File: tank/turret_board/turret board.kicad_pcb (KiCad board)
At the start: 2 copper layers, 69 x 39 mm, 22 parts, among them P1 Power, P2 IR Beacon, P3 SigIn, P4 IR Tx, P5 IR Rx, U1 LM317T, U2 pixart_ir, Y1 Crystal_4pin

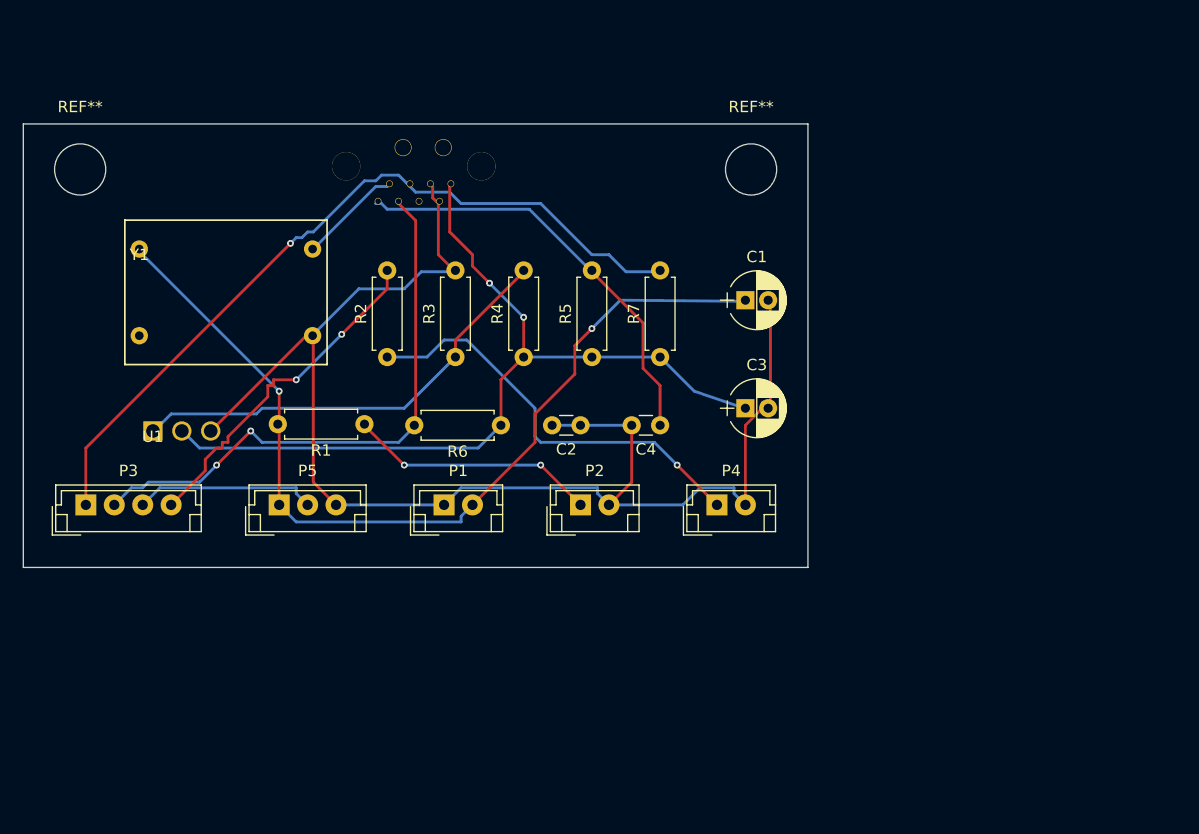
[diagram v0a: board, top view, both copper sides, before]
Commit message: main board v0.1
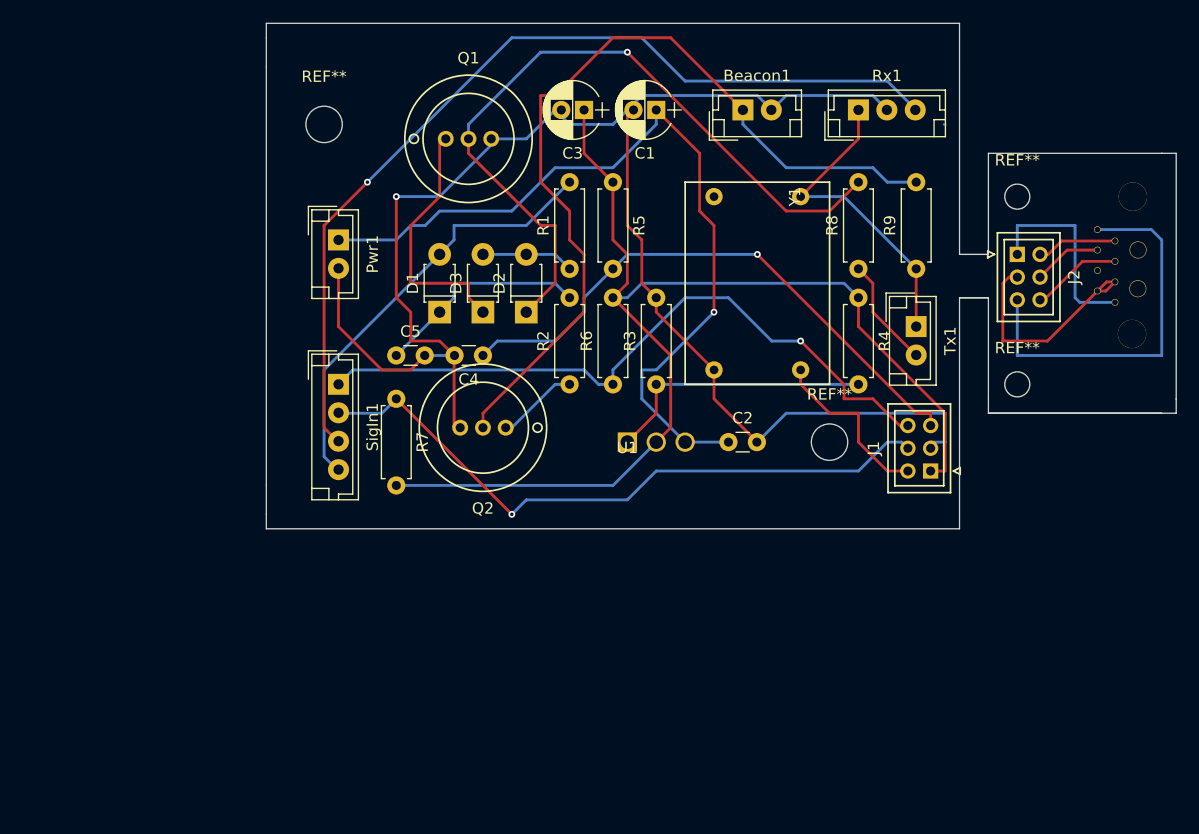
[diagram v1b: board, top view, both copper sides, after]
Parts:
- removed ?: , Tank:MIAR
- removed P1: Power, JST:JST_EH_B02B-EH-A_02x2.50mm_Straight
- removed P2: IR Beacon, JST:JST_EH_B02B-EH-A_02x2.50mm_Straight
- removed P3: SigIn, JST:JST_EH_B04B-EH-A_04x2.50mm_Straight
- removed P4: IR Tx, JST:JST_EH_B02B-EH-A_02x2.50mm_Straight
- removed P5: IR Rx, JST:JST_EH_B03B-EH-A_03x2.50mm_Straight
- removed the REF** at (150.0, 70.0)
- removed the REF** at (209.0, 70.0)
- added Beacon1: CONN_01X02, JST:JST_EH_B02B-EH-A_02x2.50mm_Straight, F.Cu at (208.3, 64.8)
- added C5: C, Capacitors_THT:C_Disc_D3.0mm_W1.6mm_P2.50mm, F.Cu at (177.8, 86.4)
- added D1: D, Diodes_THT:D_T-1_P5.08mm_Horizontal, F.Cu at (181.6, 82.5)
- added D2: D, Diodes_THT:D_T-1_P5.08mm_Horizontal, F.Cu at (189.2, 82.5)
- added D3: D, Diodes_THT:D_T-1_P5.08mm_Horizontal, F.Cu at (185.4, 82.5)
- added G***: LOGO, modules:miar_logo, B.Cu at (182.9, 71.1)
- added J1: Conn_01x06, Connectors_JAE:JAE_LY20-06P-2T_2x03x2.00mm_Straight, F.Cu at (224.8, 96.5)
- added J2: Conn_01x06, Connectors_JAE:JAE_LY20-06P-2T_2x03x2.00mm_Straight, F.Cu at (232.4, 77.5)
- added Pwr1: CONN_01X02, JST:JST_EH_B02B-EH-A_02x2.50mm_Straight, F.Cu at (172.7, 76.2)
- added Q1: Q_NPN_BCE, Transistors_OldSowjetAera:OldSowjetaera_Transistor_Type-I_SmallPads, F.Cu at (184.2, 67.3)
- added Q2: Q_NPN_BCE, Transistors_OldSowjetAera:OldSowjetaera_Transistor_Type-I_SmallPads, F.Cu at (185.4, 92.7)
- added R8: R, Resistors_THT:R_Axial_DIN0207_L6.3mm_D2.5mm_P7.62mm_Horizontal, F.Cu at (218.4, 78.7)
- added R9: R, Resistors_THT:R_Axial_DIN0207_L6.3mm_D2.5mm_P7.62mm_Horizontal, F.Cu at (223.5, 78.7)
- added REF**: MountingHole_2.2mm_M2, Mounting_Holes:MountingHole_2.2mm_M2, F.Cu at (232.4, 72.4)
- added REF**: MountingHole_3.2mm_M3, Mounting_Holes:MountingHole_3.2mm_M3, F.Cu at (171.4, 66.0)
- added REF**: MountingHole_3.2mm_M3, Mounting_Holes:MountingHole_3.2mm_M3, F.Cu at (215.9, 94.0)
- added REF**: MountingHole_2.2mm_M2, Mounting_Holes:MountingHole_2.2mm_M2, F.Cu at (232.4, 88.9)
- added Rx1: CONN_01X03, JST:JST_EH_B03B-EH-A_03x2.50mm_Straight, F.Cu at (218.4, 64.8)
- added SigIn1: CONN_01X04, JST:JST_EH_B04B-EH-A_04x2.50mm_Straight, F.Cu at (172.7, 88.9)
- added Tx1: TX, JST:JST_EH_B02B-EH-A_02x2.50mm_Straight, F.Cu at (223.5, 83.8)
- U2: footprint pixart_ir -> modules:pixart_ir
- moved Y1 58.3 mm to (213.4, 72.4), turned to 270 degrees
- moved U2 54.0 mm to (238.8, 85.1), turned to 0 degrees
- moved U1 41.7 mm to (198.1, 94.0)
- moved R4 29.9 mm to (218.4, 81.3), turned to 270 degrees
- moved C3 29.8 mm to (194.3, 64.8), turned to 180 degrees
- moved R7 23.5 mm to (177.8, 90.2), turned to 270 degrees
- moved R1 22.6 mm to (193.0, 78.7), turned to 90 degrees
- moved C1 18.5 mm to (200.7, 64.8), turned to 180 degrees
- moved R3 17.8 mm to (200.7, 88.9)
- moved C4 16.7 mm to (185.4, 86.4)
- moved R2 16.2 mm to (193.0, 88.9)
- moved R5 15.5 mm to (196.8, 71.1), turned to 270 degrees
- moved C2 13.1 mm to (207.0, 94.0), turned to 0 degrees
- moved R6 10.5 mm to (196.8, 88.9), turned to 90 degrees
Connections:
- C1 pad 2: Net-(C1-Pad2) -> GND
- C2 pad 1: Net-(C1-Pad2) -> Net-(C1-Pad1)
- C2 pad 2: Net-(C1-Pad2) -> GND
- C3 pad 1: +3V3 -> 3.3V
- C3 pad 2: Net-(C1-Pad2) -> GND
- C4 pad 1: Net-(C4-Pad1) -> RESET
- C4 pad 2: Net-(C1-Pad2) -> GND
- R1 pad 2: Net-(C1-Pad1) -> IRSig
- R3 pad 2: Net-(C1-Pad2) -> GND
- R4 pad 1: +3V3 -> 3.3V
- R5 pad 1: +3V3 -> 3.3V
- R5 pad 2: Net-(C4-Pad1) -> RESET
- R6 pad 1: +3V3 -> SLC
- R6 pad 2: Net-(P3-Pad2) -> 3.3V
- R7 pad 1: +3V3 -> SDA
- R7 pad 2: Net-(P3-Pad1) -> 3.3V
- U1 pad 2: +3V3 -> 3.3V
- U1 pad 3: Net-(C1-Pad2) -> Net-(C1-Pad1)
- U2 pad 1: +3V3 -> Net-(J2-Pad1)
- U2 pad 2: Net-(C1-Pad2) -> Net-(J2-Pad2)
- U2 pad 3: Net-(C1-Pad2) -> Net-(J2-Pad2)
- U2 pad 5: Net-(P3-Pad1) -> Net-(J2-Pad6)
- U2 pad 6: Net-(P3-Pad2) -> Net-(J2-Pad5)
- U2 pad 7: Net-(U2-Pad7) -> Net-(J2-Pad4)
- U2 pad 8: Net-(C4-Pad1) -> Net-(J2-Pad3)
- Y1 pad 14: Net-(C1-Pad1) -> 5V
- Y1 pad 7: Net-(C1-Pad2) -> GND
- Y1 pad 8: Net-(U2-Pad7) -> Net-(J1-Pad4)
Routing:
- net GND: track 0.00 -> 151.4 mm, vias 0 -> 1
- net Net-(C1-Pad2): track 127.5 -> 0.00 mm
- net 3.3V: track 0.00 -> 100.7 mm
- net Net-(Rx1-Pad3): track 0.00 -> 81.3 mm, vias 0 -> 1
- net +3V3: track 75.7 -> 0.00 mm, vias 2 -> 0
- net Beacon: track 0.00 -> 75.6 mm
- net Net-(P3-Pad1): track 69.6 -> 0.00 mm, vias 1 -> 0
- net Net-(D2-Pad1): track 0.00 -> 65.2 mm, vias 0 -> 1
- net SLC: track 0.00 -> 60.5 mm, vias 0 -> 1
- net SDA: track 0.00 -> 57.7 mm, vias 0 -> 1
- net Net-(P3-Pad2): track 50.8 -> 0.00 mm, vias 2 -> 0
- net RESET: track 0.00 -> 50.7 mm, vias 0 -> 1
- net IRSig: track 0.00 -> 38.7 mm
- net Net-(C4-Pad1): track 38.0 -> 0.00 mm
- net Net-(J2-Pad3): track 0.00 -> 33.8 mm
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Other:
- board size 69 x 39 mm -> 80 x 44.4 mm
- board text added: "Turret Board v0.3 Laser Tag Robot Tank M.I.A.R. Labs nick.groesz@gmail.com"
- board text removed: "Turret Board v0.2 Laser Bot M.I.A.R. Labs"

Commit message: interim
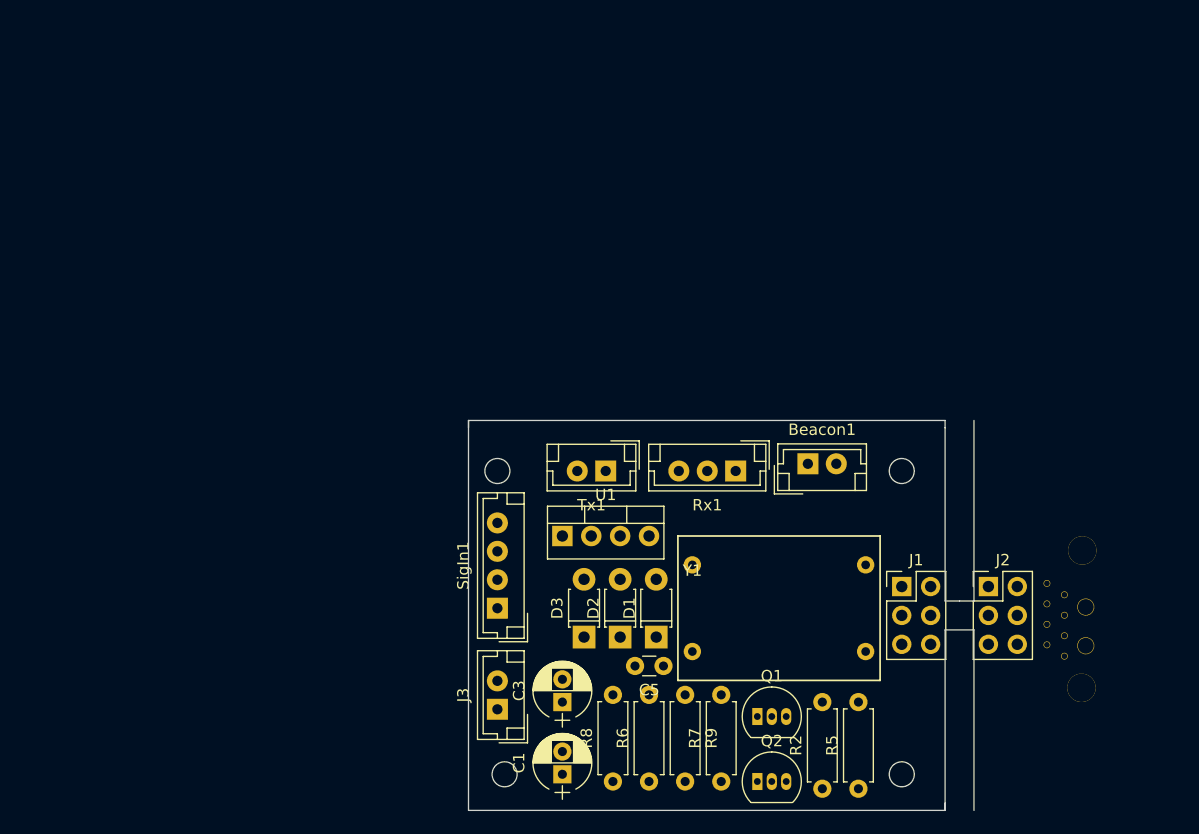
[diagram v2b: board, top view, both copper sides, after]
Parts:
- removed C2, C4: C, Capacitors_THT:C_Disc_D3.0mm_W1.6mm_P2.50mm
- removed G***: LOGO, modules:miar_logo
- removed Pwr1: CONN_01X02, JST:JST_EH_B02B-EH-A_02x2.50mm_Straight
- removed R1, R3, R4: R, Resistors_THT:R_Axial_DIN0207_L6.3mm_D2.5mm_P7.62mm_Horizontal
- removed the REF** at (232.4, 72.4)
- removed the REF** at (171.4, 66.0)
- removed the REF** at (215.9, 94.0)
- removed the REF** at (232.4, 88.9)
- added J3: Conn_01x02_Male, JST:JST_EH_B02B-EH-A_02x2.50mm_Straight, F.Cu at (186.7, 117.5)
- added REF**: MountingHole_2.2mm_M2, Mounting_Holes:MountingHole_2.2mm_M2, F.Cu at (186.7, 96.5)
- added REF**: MountingHole_2.2mm_M2, Mounting_Holes:MountingHole_2.2mm_M2, F.Cu at (187.3, 123.2)
- added REF**: MountingHole_2.2mm_M2, Mounting_Holes:MountingHole_2.2mm_M2, F.Cu at (222.2, 96.5)
- added REF**: MountingHole_2.2mm_M2, Mounting_Holes:MountingHole_2.2mm_M2, F.Cu at (222.2, 123.2)
- J1, J2: footprint Connectors_JAE:JAE_LY20-06P-2T_2x03x2.00mm_Straight -> Pin_Headers:Pin_Header_Straight_2x03_Pitch2.54mm
- Q1, Q2: value Q_NPN_BCE -> 2N3904; footprint Transistors_OldSowjetAera:OldSowjetaera_Transistor_Type-I_SmallPads -> TO_SOT_Packages_THT:TO-92_Inline_Narrow_Oval
- U1: value LM317T -> KA378R33; footprint Tank:LM317T -> TO_SOT_Packages_THT:TO-220-4_Vertical
- moved C1 59.0 mm to (192.4, 123.2), turned to 90 degrees
- moved R5 57.5 mm to (218.4, 124.5), turned to 90 degrees
- moved Q1 56.8 mm to (209.6, 118.1)
- moved C3 52.1 mm to (192.4, 116.8), turned to 90 degrees
- moved R8 50.0 mm to (196.8, 123.8)
- moved R7 44.1 mm to (206.4, 123.8), turned to 90 degrees
- moved R9 42.6 mm to (203.2, 116.2), turned to 270 degrees
- moved R2 41.9 mm to (215.3, 124.5)
- moved Q2 39.4 mm to (209.6, 123.8), turned to 0 degrees
- moved C5 36.0 mm to (201.3, 113.7), turned to 180 degrees
- moved R6 35.1 mm to (200.0, 123.8)
- moved D1 34.3 mm to (200.7, 111.1)
- moved Y1 33.8 mm to (203.8, 104.8), turned to 0 degrees
- moved Rx1 33.5 mm to (207.6, 96.5), turned to 180 degrees
- moved Beacon1 31.6 mm to (214.0, 95.9)
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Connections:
- D2 pad 2: Net-(D2-Pad2) -> IRSig
- D3 pad 2: Net-(D2-Pad2) -> IRSig
- J1 pad 3: RESET -> GND
- Q1 pad 1: Net-(D3-Pad1) -> GND
- Q1 pad 2: Net-(D2-Pad1) -> Net-(D3-Pad1)
- Q1 pad 3: GND -> Net-(D2-Pad1)
- Q2 pad 1: Net-(Q2-Pad1) -> GND
- Q2 pad 2: Beacon -> Net-(Q2-Pad2)
- Q2 pad 3: GND -> Beacon
- R2 pad 1: Net-(Q2-Pad1) -> Net-(Q2-Pad2)
- R5 pad 2: RESET -> GND
- Rx1 pad 3: Net-(Rx1-Pad3) -> IRRx
- SigIn1 pad 3: Net-(Rx1-Pad3) -> IRSig
- SigIn1 pad 4: IRSig -> IRRx
- U1 pad 1: Net-(R3-Pad1) -> Net-(C1-Pad1)
- U1 pad 3: Net-(C1-Pad1) -> GND
- Y1 pad 14: 5V -> 3.3V
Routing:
- net GND: track 151.4 -> 0.00 mm, vias 1 -> 0
- net 3.3V: track 100.7 -> 0.00 mm
- net Net-(Rx1-Pad3): track 81.3 -> 0.00 mm, vias 1 -> 0
- net Beacon: track 75.6 -> 0.00 mm
- net Net-(C1-Pad1): track 73.5 -> 0.00 mm, vias 1 -> 0
- net Net-(D2-Pad1): track 65.2 -> 0.00 mm, vias 1 -> 0
- net SLC: track 60.5 -> 0.00 mm, vias 1 -> 0
- net SDA: track 57.7 -> 0.00 mm, vias 1 -> 0
- net RESET: track 50.7 -> 0.00 mm, vias 1 -> 0
- net IRSig: track 38.7 -> 0.00 mm
- net Net-(J2-Pad3): track 33.8 -> 0.00 mm
- net 5V: track 27.6 -> 0.00 mm
- net Net-(R3-Pad1): track 23.9 -> 0.00 mm
- net Net-(D3-Pad1): track 22.4 -> 0.00 mm
- net Net-(J2-Pad2): track 20.5 -> 0.00 mm
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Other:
- board size 80 x 44.4 mm -> 44.4 x 34.3 mm
- board text removed: "Turret Board v0.3 Laser Tag Robot Tank M.I.A.R. Labs nick.groesz@gmail.com"
